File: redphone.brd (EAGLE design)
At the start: 146 x 65 mm, 307 parts, among them IC1 EP4CE6E22, IC10 MPU9250, IC11 PCA9633TK, IC12 HDC1000, IC13 TPS63000, IC14 24LC256, IC16 EPCS4SI8N, IC18 WM8903, IC19 AT25SF041, IC2 STM32F429ZIT, IC20 MP34DT01, IC21 PT4181, IC22 MAX8903A, IC23 NRF24L01, IC24 BME280, IC25 APDS-9960, IC26 DS18B20U, IC27 MC-1010-G, IC28 MAX2659, IC3 MT48LC16M16A2TG, IC4 MAX8815A, IC5 LP3990TL, IC6 LP3990TL, IC7 TPS63001, IC8 ESP8266, IC9 SIM800C, Q1 IRLML6402, Q2 NTA4153NT1G, Q3 BCR133W, Q4 NTA4153NT1G, Q5 NTA4153NT1G, Q6 IRLML6402, Q7 16MHz, Q8 NTA4153NT1G, SW1 PWR, SW2 CAM, SW3 VOL+, SW4 VOL-, X1 MICRO_SIM_SDS, X10 AUDIO-JACKSMD, X13 OV2640, X14 UFL, X16 USB, X18 FPC_I9500_BAT_CON, X3 RM68120_LCD, X5 LG_P715_TS, Y1 2.4Ghz, Y3 2.4Ghz, Y4 GSM_PCB, Y5 2.4Ghz

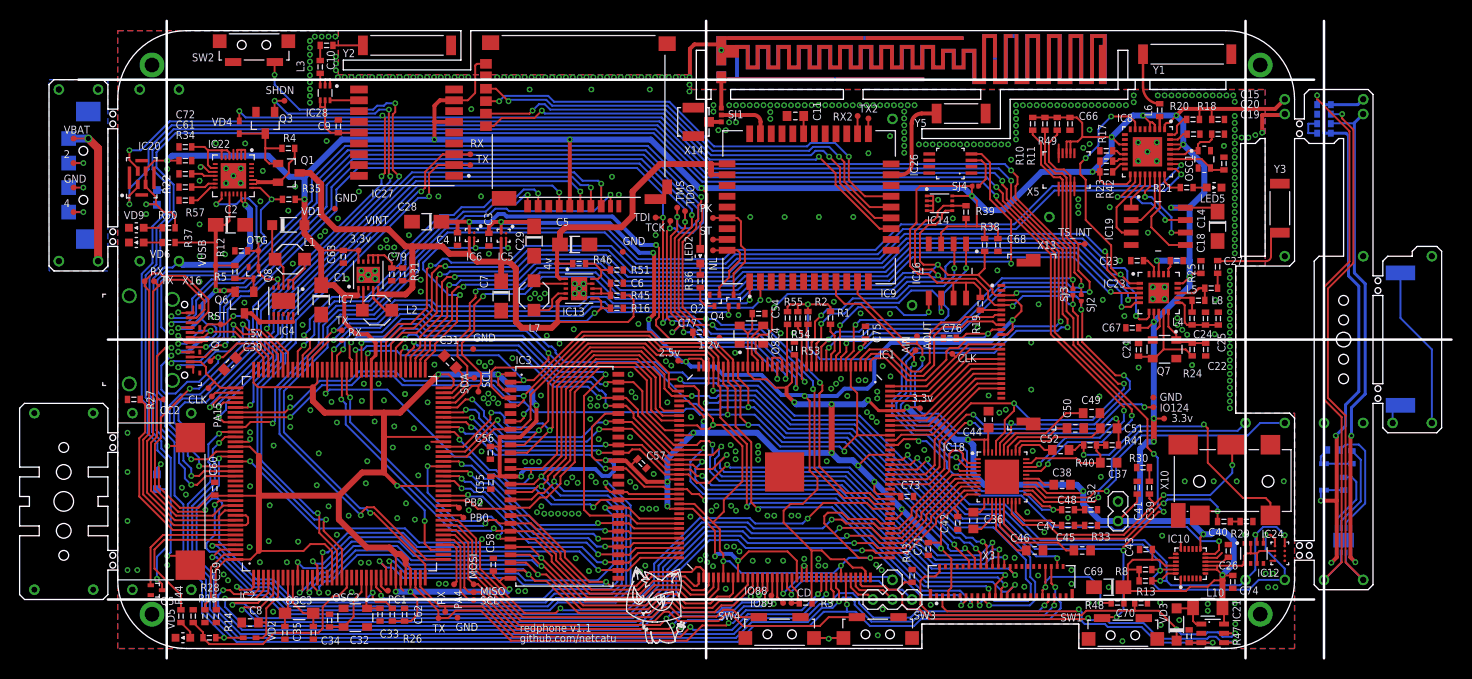
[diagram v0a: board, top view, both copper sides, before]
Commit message: fix pkg of gps lna, cap & res values fix, drc fix
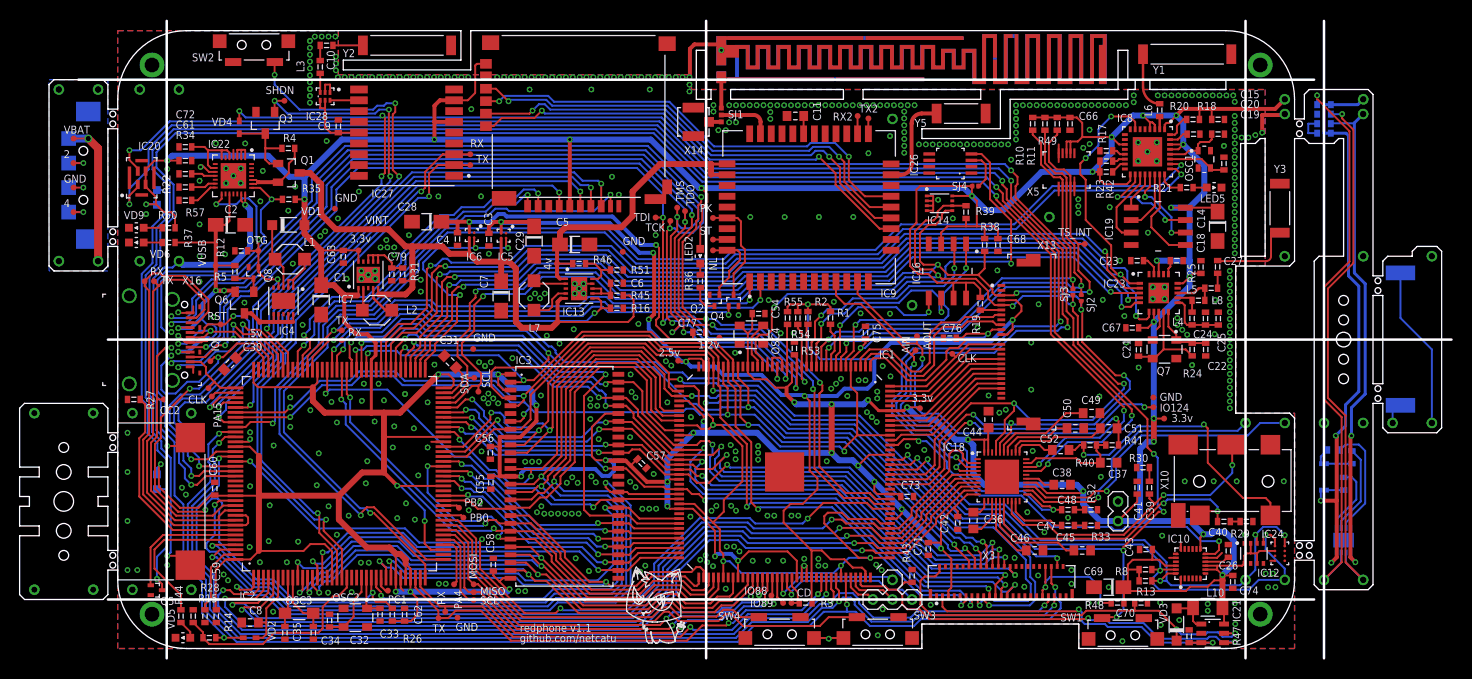
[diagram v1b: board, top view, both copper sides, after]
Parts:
- C10: value (none) -> 470p
- L3: value (none) -> 6.8uH
- R46: value 1M -> 1.5M
- R51: value 220k -> 215k
- moved IC28 0.35 mm to (21.1, 56.3)
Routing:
- net N$72: track 1.25 -> 1.95 mm
